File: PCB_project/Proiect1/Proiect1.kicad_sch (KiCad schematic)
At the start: 29 parts, among them J1 Conn_01x01_Pin, J2 Conn_01x01_Pin, J3 Conn_01x01_Pin, J4 Conn_01x01_Pin, Q1 BS170FTA, Q10 BS170FTA, Q11 BS250FTA, Q12 BS170FTA, Q13 BS170FTA, Q2 BS170FTA, Q3 BS250FTA, Q4 BS170FTA, Q5 BS250FTA, Q6 BS170FTA, Q7 BS170FTA, Q8 BS250FTA, Q9 BS250FTA

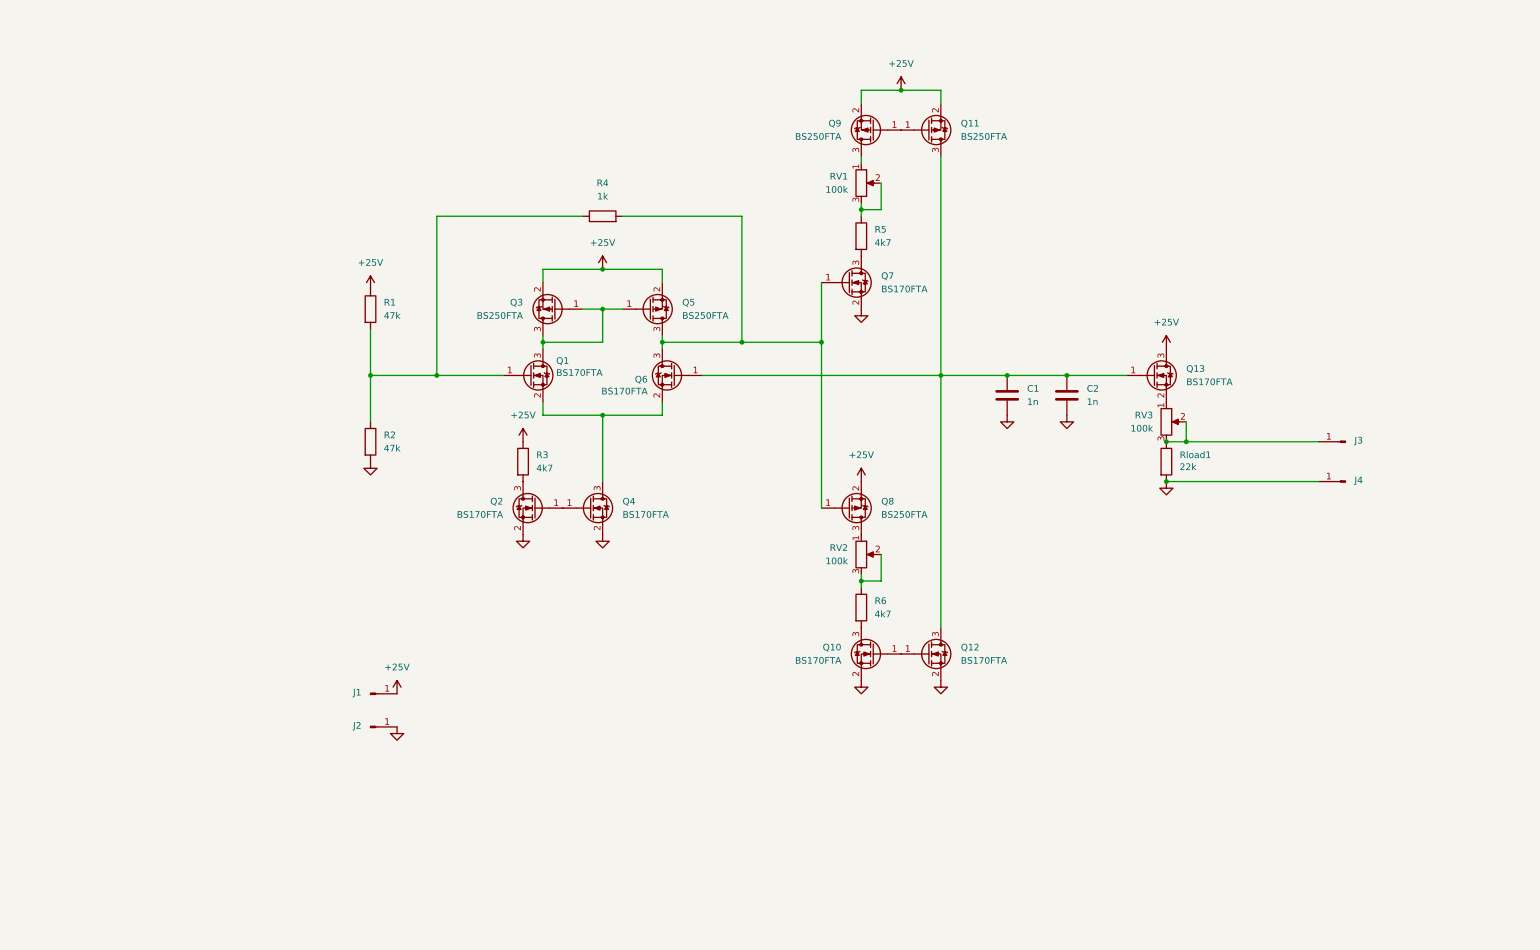
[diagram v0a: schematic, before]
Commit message: Started new PCB
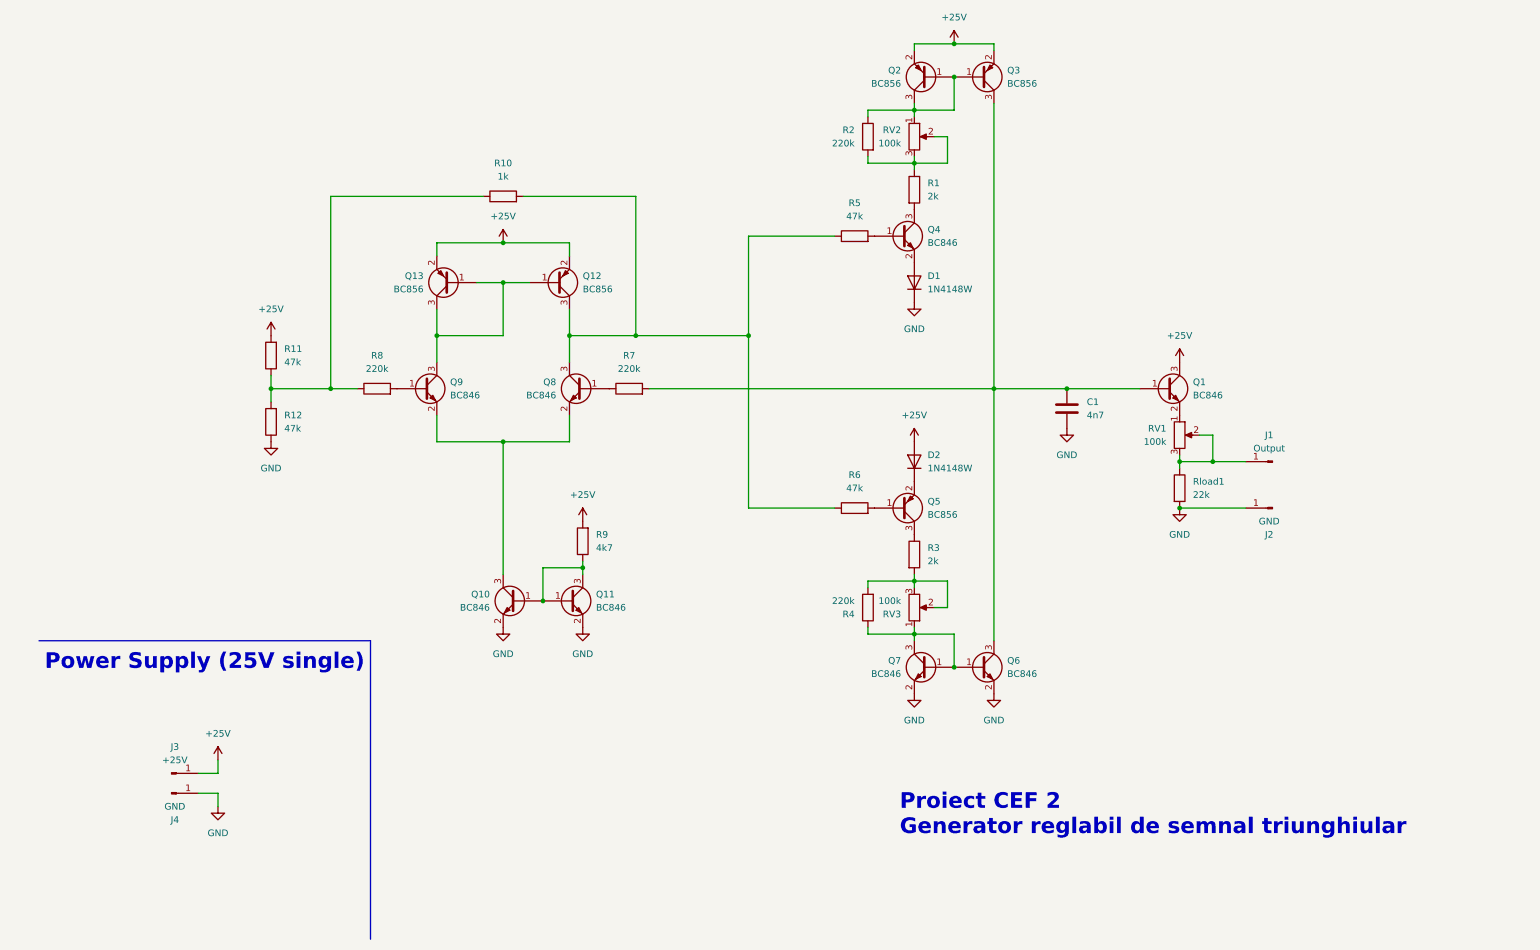
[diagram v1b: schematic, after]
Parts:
- removed C2: 1n, Capacitor_SMD:C_0805_2012Metric, symbol Device:C
- removed Q1, Q10, Q12, Q13, Q2, Q4, Q6, Q7: BS170FTA, Package_TO_SOT_SMD:SOT-23, symbol Transistor_FET:BS170F
- removed Q11, Q3, Q5, Q8, Q9: BS250FTA, Package_TO_SOT_SMD:SOT-23, symbol Transistor_FET:BS250
- added D1, D2: 1N4148W, Diode_SMD:D_0805_2012Metric, symbol Diode:1N4148W
- added Q1, Q10, Q11, Q4, Q6, Q7, Q8, Q9: BC846, Package_TO_SOT_SMD:SOT-23, symbol Transistor_BJT:BC846
- added Q12, Q13, Q2, Q3, Q5: BC856, Package_TO_SOT_SMD:SOT-23, symbol Transistor_BJT:BC856
- added R10: 1k, Resistor_SMD:R_0805_2012Metric, symbol Device:R
- added R11, R12: 47k, Resistor_SMD:R_0805_2012Metric, symbol Device:R
- added R7, R8: 220k, Resistor_SMD:R_0805_2012Metric, symbol Device:R
- added R9: 4k7, Resistor_SMD:R_0805_2012Metric, symbol Device:R
- C1: value 1n -> 4n7; TME https://www.tme.eu/ro/en/details/grm2165c2a102ja01d/mlcc-sm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 -> (none)
- J1: value Conn_01x01_Pin -> Output; footprint Connector_PinHeader_2.54mm:PinHeader_1x01_P2.54mm_Vertical -> Connector_PinHeader_2.00mm:PinHeader_1x01_P2.00mm_Vertical
- J2, J4: value Conn_01x01_Pin -> GND; footprint Connector_PinHeader_2.54mm:PinHeader_1x01_P2.54mm_Vertical -> Connector_PinHeader_2.00mm:PinHeader_1x01_P2.00mm_Vertical
- J3: value Conn_01x01_Pin -> +25V; footprint Connector_PinHeader_2.54mm:PinHeader_1x01_P2.54mm_Vertical -> Connector_PinHeader_2.00mm:PinHeader_1x01_P2.00mm_Vertical
- R1: value 47k -> 2k; TME https://www.tme.eu/ro/en/details/erj6geyj473v/smd-resistors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 -> (none)
- R2: value 47k -> 220k; TME https://www.tme.eu/ro/en/details/erj6geyj473v/smd-resistors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 -> (none)
- R3: value 4k7 -> 2k; TME https://www.tme.eu/ro/en/details/erjp06j472v/smd-resistors/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 -> (none)
- R4: value 1k -> 220k; TME https://www.tme.eu/ro/en/details/rc0805fr-071k/smd-resistor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 -> (none)
- R5, R6: value 4k7 -> 47k; TME https://www.tme.eu/ro/en/details/erjp06j472v/smd-resistors/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 -> (none)
- RV1, RV2, RV3: footprint zCustom_Footprints:3361P_1 -> Potentiometer_SMD:Potentiometer_Vishay_TS53YL_Vertical; TME https://www.tme.eu/ro/en/details/3361p-1-104glf/single-turn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 -> (none)
- Rload1: TME https://www.tme.eu/ro/en/details/erj6geyj223v/smd-resistors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 -> (none)
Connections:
- net +25V: now also J3.1 (Pin_1), D2.2 (A), Q1.3 (C), Q12.2 (E), Q13.2 (E), Q2.2 (E), Q3.2 (E), R11.2, R9.2; no longer J1.1 (Pin_1), R1.1, R3.1
- net GND: now also D1.1 (K), Q10.2 (E), Q11.2 (E), Q6.2 (E), Q7.2 (E), R12.1; no longer R2.2
- net at C1.1: now also Q1.1 (B), Q3.3 (C), Q6.3 (C), R7.2
- net at R4.2: now also R3.2, RV3.2, RV3.3
- net at RV2.1: now also R2.1, Q2.1 (B), Q2.3 (C), Q3.1 (B)
- net at RV2.2, RV2.3: now also R1.1, R2.2; no longer R6.1
- net at RV1.1: now also Q1.2 (E)
- net at RV1.2, RV1.3: now also J1.1 (Pin_1), Rload1.1; no longer R5.1
- net at R5.2: now also Q4.1 (B)
- net at RV3.1: now also R4.1, Q6.1 (B), Q7.1 (B), Q7.3 (C)
- net at R6.2: now also Q5.1 (B)
- new net: Q12.3 (C), Q8.3 (C), R10.2, R5.1, R6.1
- new net: Q8.1 (B), R7.1
- new net: Q10.3 (C), Q8.2 (E), Q9.2 (E)
- new net: D2.1 (K), Q5.2 (E)
- new net: Q5.3 (C), R3.1
- new net: Q10.1 (B), Q11.1 (B), Q11.3 (C), R9.1
- new net: R10.1, R11.1, R12.2, R8.1
- new net: Q4.3 (C), R1.2
- new net: Q12.1 (B), Q13.1 (B), Q13.3 (C), Q9.3 (C)
- new net: D1.2 (A), Q4.2 (E)
- new net: Q9.1 (B), R8.2
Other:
- note added: "Power Supply (25V single)"
- note added: "Proiect CEF 2 Generator reglabil de semnal triunghiular"
- company: (none) -> Fratu-Halunga Theodor (434C)
- title: (none) -> Proiect CEF 2 - Generator reglabil de semnal triunghiular
